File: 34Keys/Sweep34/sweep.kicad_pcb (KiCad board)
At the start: 2 copper layers, 110 x 88.6 mm, 21 parts, among them J1 MJ-4PP-9, SW10 SW_PUSH, SW11 SW_PUSH, SW12 SW_PUSH, SW14 SW_PUSH, SW15 SW_PUSH, SW16 SW_PUSH, SW17 SW_PUSH, SW18 SW_PUSH, SW2 SW_PUSH, SW20 SW_PUSH, SW21 SW_PUSH, SW3 SW_PUSH, SW4 SW_PUSH, SW5 SW_PUSH, SW6 SW_PUSH, SW8 SW_PUSH, SW9 SW_PUSH, U1 ProMicro

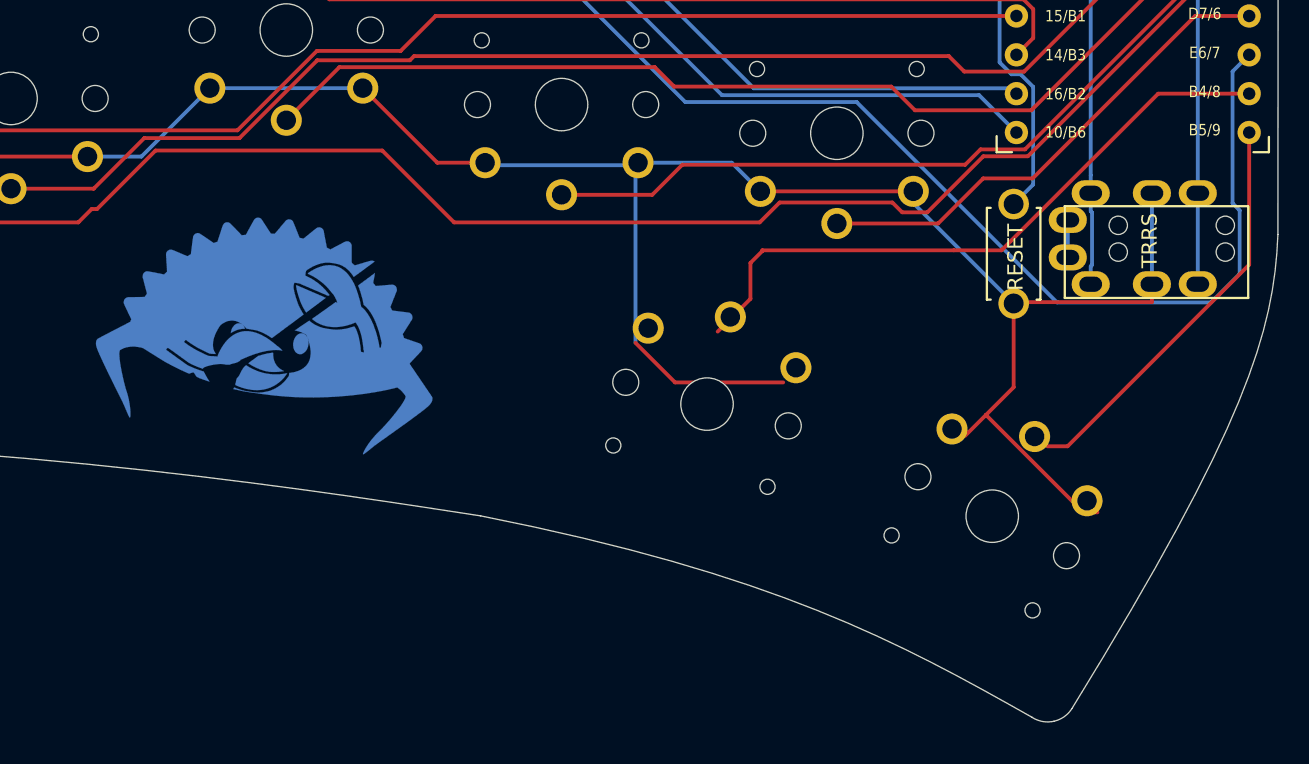
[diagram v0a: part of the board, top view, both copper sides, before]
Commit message: let's get these thumbs something like ferris
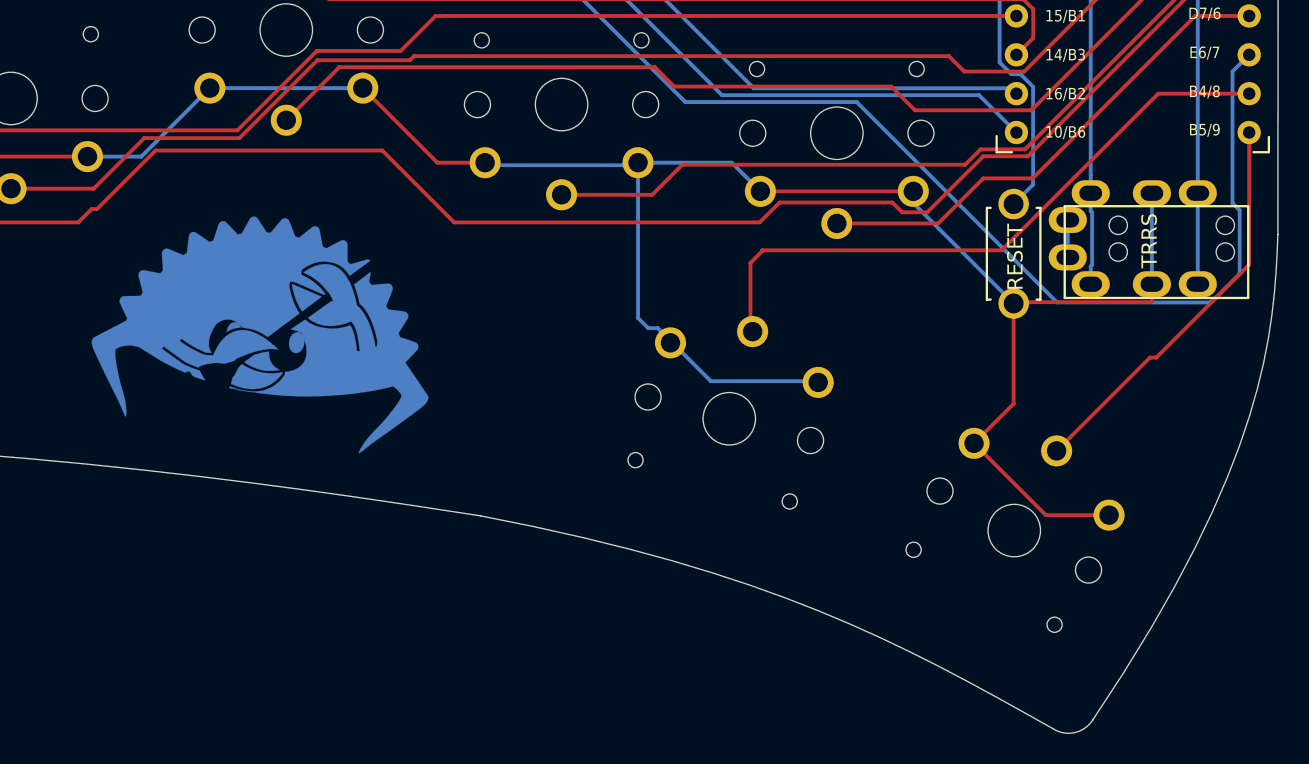
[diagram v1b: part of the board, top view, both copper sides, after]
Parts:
- moved SW20 1.74 mm to (109.0, 85.1)
- moved SW21 1.72 mm to (127.6, 92.4)
- moved G*** 0.28 mm to (79.8, 80.3)
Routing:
- net GND: track 393.6 -> 396.0 mm
- net Net-(U1-Pad11): track 42.6 -> 41.7 mm
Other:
- board size 110 x 88.6 mm -> 110 x 89.3 mm
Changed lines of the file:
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@@
   )
   (module Kailh:SW_PG1350_reversible_b2 (layer B.Cu)
-    (at 126.16 91.46 332)
+    (at 127.6 92.4 332)
     (descr "Kailh \"Choc\" PG1350 keyswitch, able to be mounted on front or back of PCB")
     (tags kailh,choc)
@@
   )
   (module Kailh:SW_PG1350_reversible_b2 (layer B.Cu)
-    (at 107.51 84.13 345)
+    (at 108.966 85.09 345)
     (descr "Kailh \"Choc\" PG1350 keyswitch, able to be mounted on front or back of PCB")
     (tags kailh,choc)
@@
   )
   (module Kailh:ferris_broom (layer B.Cu)
-    (at 80.07 80.4 171)
+    (at 79.8 80.33 171)
     (fp_text reference G*** (at 0 0 351) (layer B.SilkS) hide
       (effects (font (size 1.524 1.524) (thickness 0.3)) (justify mirror))
@@
   (gr_curve (pts (xy 144.87 34.010455) (xy 144.870889 33.819247) (xy 144.795513 33.637251) (xy 144.655943 33.499545)) (layer Edge.Cuts) (width 0.011328))
   (gr_curve (pts (xy 125.294806 23.859172) (xy 125.294794 23.580455) (xy 125.132917 23.327117) (xy 124.9 23.22)) (layer Edge.Cuts) (width 0.011328))
-  (gr_curve (pts (xy 130.186173 104.869608) (xy 130.675764 104.762323) (xy 131.102064 104.463579) (xy 131.37 104.04)) (layer Edge.Cuts) (width 0.011328))
-  (gr_curve (pts (xy 128.763902 104.611077) (xy 129.184419 104.883795) (xy 129.696582 104.976892) (xy 130.186173 104.869608)) (layer Edge.Cuts) (width 0.011328))
+  (gr_curve (pts (xy 131.55 105.61) (xy 132.039591 105.502715) (xy 132.465891 105.203971) (xy 132.73 104.79)) (layer Edge.Cuts) (width 0.011328))
+  (gr_curve (pts (xy 130.127729 105.351469) (xy 130.548246 105.624187) (xy 131.060409 105.717284) (xy 131.55 105.61)) (layer Edge.Cuts) (width 0.011328))
   (gr_curve (pts (xy 34.833624 84.713423) (xy 34.87005 85.754071) (xy 35.733715 86.573551) (xy 36.77484 86.555327)) (layer Edge.Cuts) (width 0.011328))
-  (gr_curve (pts (xy 128.763902 104.611077) (xy 120.073417 99.705624) (xy 111.98 95.25) (xy 92.71 91.44)) (layer Edge.Cuts) (width 0.011328))
+  (gr_curve (pts (xy 130.127729 105.351469) (xy 120.073417 99.705624) (xy 111.83 95.11) (xy 92.71 91.44)) (layer Edge.Cuts) (width 0.011328))
   (gr_line (start 125.3 31.44) (end 125.294806 23.859172) (layer Edge.Cuts) (width 0.011328))
   (gr_curve (pts (xy 124.9 23.22) (xy 111.07043 20.337524) (xy 96.846186 17.334305) (xy 84.254525 16.504695)) (layer Edge.Cuts) (width 0.011328))
@@
   (gr_curve (pts (xy 80.49 16.32) (xy 63.51 16.12) (xy 48.01 22.1) (xy 36.11 33.02)) (layer Edge.Cuts) (width 0.011328))
   (gr_line (start 144.87 34.010455) (end 144.84 73.04) (layer Edge.Cuts) (width 0.011328))
-  (gr_curve (pts (xy 131.37 104.04) (xy 142.702381 85.610668) (xy 144.590037 79.411298) (xy 144.84 73.04)) (layer Edge.Cuts) (width 0.011328))
+  (gr_curve (pts (xy 132.73 104.79) (xy 144.15 87.83) (xy 144.590037 79.411298) (xy 144.84 73.04)) (layer Edge.Cuts) (width 0.011328))
   (segment (start 142.9614 53.672) (end 139.966 53.672) (width 0.25) (layer F.Cu) (net 1))
   (segment (start 139.966 53.672) (end 128.7186 64.9194) (width 0.25) (layer F.Cu) (net 1))
@@
   (segment (start 49 80.175) (end 39 80.175) (width 0.25) (layer F.Cu) (net 5))
   (segment (start 102.8339 68.5111) (end 103 68.345) (width 0.25) (layer B.Cu) (net 5))
-  (segment (start 102.8339 80.1254) (end 102.8339 68.5111) (width 0.25) (layer B.Cu) (net 5))
   (segment (start 102.8339 68.5111) (end 93.1661 68.5111) (width 0.25) (layer B.Cu) (net 5))
   (segment (start 93.1661 68.5111) (end 93 68.345) (width 0.25) (layer B.Cu) (net 5))
@@
   (segment (start 88.2995 46.6395) (end 88.2995 46.47) (width 0.25) (layer B.Cu) (net 5))
   (segment (start 88.2995 46.47) (end 85 46.47) (width 0.25) (layer B.Cu) (net 5))
-  (segment (start 125.7506 84.8384) (end 124.3799 86.2091) (width 0.25) (layer F.Cu) (net 5))
-  (segment (start 127.56 77.55) (end 127.56 83.029) (width 0.25) (layer F.Cu) (net 5))
-  (segment (start 127.56 83.029) (end 125.7506 84.8384) (width 0.25) (layer F.Cu) (net 5))
-  (segment (start 125.7506 84.8384) (end 132.1213 91.2091) (width 0.25) (layer F.Cu) (net 5))
-  (segment (start 132.1213 91.2091) (end 133.0401 91.2091) (width 0.25) (layer F.Cu) (net 5))
   (segment (start 136.6 77.4653) (end 127.6447 77.4653) (width 0.25) (layer F.Cu) (net 5))
   (segment (start 127.6447 77.4653) (end 127.56 77.55) (width 0.25) (layer F.Cu) (net 5))
@@
   (segment (start 75 63.47) (end 70.525 67.945) (width 0.25) (layer B.Cu) (net 5))
   (segment (start 70.525 67.945) (end 67 67.945) (width 0.25) (layer B.Cu) (net 5))
-  (segment (start 112.4931 82.7136) (end 105.4221 82.7136) (width 0.25) (layer F.Cu) (net 5))
-  (segment (start 105.4221 82.7136) (end 102.8339 80.1254) (width 0.25) (layer F.Cu) (net 5))
   (segment (start 142.9614 43.512) (end 140.4214 40.972) (width 0.25) (layer F.Cu) (net 5))
   (segment (start 140.4214 40.972) (end 127.7414 40.972) (width 0.25) (layer F.Cu) (net 5))
@@
   (segment (start 136.6 76.29) (end 136.6 77.4653) (width 0.25) (layer F.Cu) (net 5))
   (segment (start 136.6 76.29) (end 136.6 70.34) (width 0.25) (layer B.Cu) (net 5))
+  (segment (start 103 78.501504) (end 103.663883 79.165387) (width 0.25) (layer B.Cu) (net 5))
+  (segment (start 103 68.345) (end 103 78.501504) (width 0.25) (layer B.Cu) (net 5))
+  (segment (start 127.56 84.106695) (end 124.969254 86.697441) (width 0.25) (layer F.Cu) (net 5))
+  (segment (start 127.56 77.55) (end 127.56 84.106695) (width 0.25) (layer F.Cu) (net 5))
+  (segment (start 129.66397 91.392157) (end 133.79873 91.392157) (width 0.25) (layer F.Cu) (net 5))
+  (segment (start 124.969254 86.697441) (end 129.66397 91.392157) (width 0.25) (layer F.Cu) (net 5))
+  (segment (start 107.762073 82.633577) (end 105.173883 80.045387) (width 0.25) (layer B.Cu) (net 5))
+  (segment (start 114.833142 82.633577) (end 107.762073 82.633577) (width 0.25) (layer B.Cu) (net 5))
+  (segment (start 104.293883 79.165387) (end 105.173883 80.045387) (width 0.25) (layer B.Cu) (net 5))
+  (segment (start 103.663883 79.165387) (end 104.293883 79.165387) (width 0.25) (layer B.Cu) (net 5))
   (segment (start 132.6 69.1647) (end 132.6 50.9106) (width 0.25) (layer B.Cu) (net 6))
   (segment (start 132.6 50.9106) (end 127.7414 46.052) (width 0.25) (layer B.Cu) (net 6))
@@
   (segment (start 108.4899 63.9299) (end 98 53.44) (width 0.25) (layer B.Cu) (net 21))
   (segment (start 142.9614 66.372) (end 142.9614 75.0149) (width 0.25) (layer F.Cu) (net 22))
-  (segment (start 142.9614 75.0149) (end 131.0858 86.8905) (width 0.25) (layer F.Cu) (net 22))
-  (segment (start 131.0858 86.8905) (end 129.76 86.8905) (width 0.25) (layer F.Cu) (net 22))
-  (segment (start 137.0102 63.832) (end 142.9614 63.832) (width 0.25) (layer F.Cu) (net 23))
-  (segment (start 127.4086 73.4336) (end 137.0102 63.832) (width 0.25) (layer F.Cu) (net 23))
-  (segment (start 110.35 77.24807) (end 108.207032 79.391038) (width 0.25) (layer F.Cu) (net 23))
+  (segment (start 142.9614 75.0149) (end 136.88815 81.08815) (width 0.25) (layer F.Cu) (net 22))
+  (segment (start 136.472341 81.08815) (end 130.369882 87.190609) (width 0.25) (layer F.Cu) (net 22))
+  (segment (start 136.88815 81.08815) (end 136.472341 81.08815) (width 0.25) (layer F.Cu) (net 22))
+  (segment (start 110.35 74.9) (end 110.35 79.114006) (width 0.25) (layer F.Cu) (net 23))
+  (segment (start 110.35 79.114006) (end 110.547032 79.311038) (width 0.25) (layer F.Cu) (net 23))
+  (segment (start 142.9614 63.832) (end 137.0102 63.832) (width 0.25) (layer F.Cu) (net 23))
   (segment (start 111.125 74.125) (end 110.35 74.9) (width 0.25) (layer F.Cu) (net 23))
+  (segment (start 137.0102 63.832) (end 126.7672 74.075) (width 0.25) (layer F.Cu) (net 23))
+  (segment (start 126.7672 74.075) (end 111.125 74.075) (width 0.25) (layer F.Cu) (net 23))
   (segment (start 111.125 74.075) (end 111.125 74.125) (width 0.25) (layer F.Cu) (net 23))
-  (segment (start 111.125 74.075) (end 123.65 74.075) (width 0.25) (layer F.Cu) (net 23))
-  (segment (start 110.35 74.9) (end 110.35 77.24807) (width 0.25) (layer F.Cu) (net 23))
-  (segment (start 126.7672 74.075) (end 126.8711 73.9711) (width 0.25) (layer F.Cu) (net 23))
-  (segment (start 123.65 74.075) (end 126.7672 74.075) (width 0.25) (layer F.Cu) (net 23))
-  (segment (start 126.8711 73.9711) (end 127.4086 73.4336) (width 0.25) (layer F.Cu) (net 23))
 )

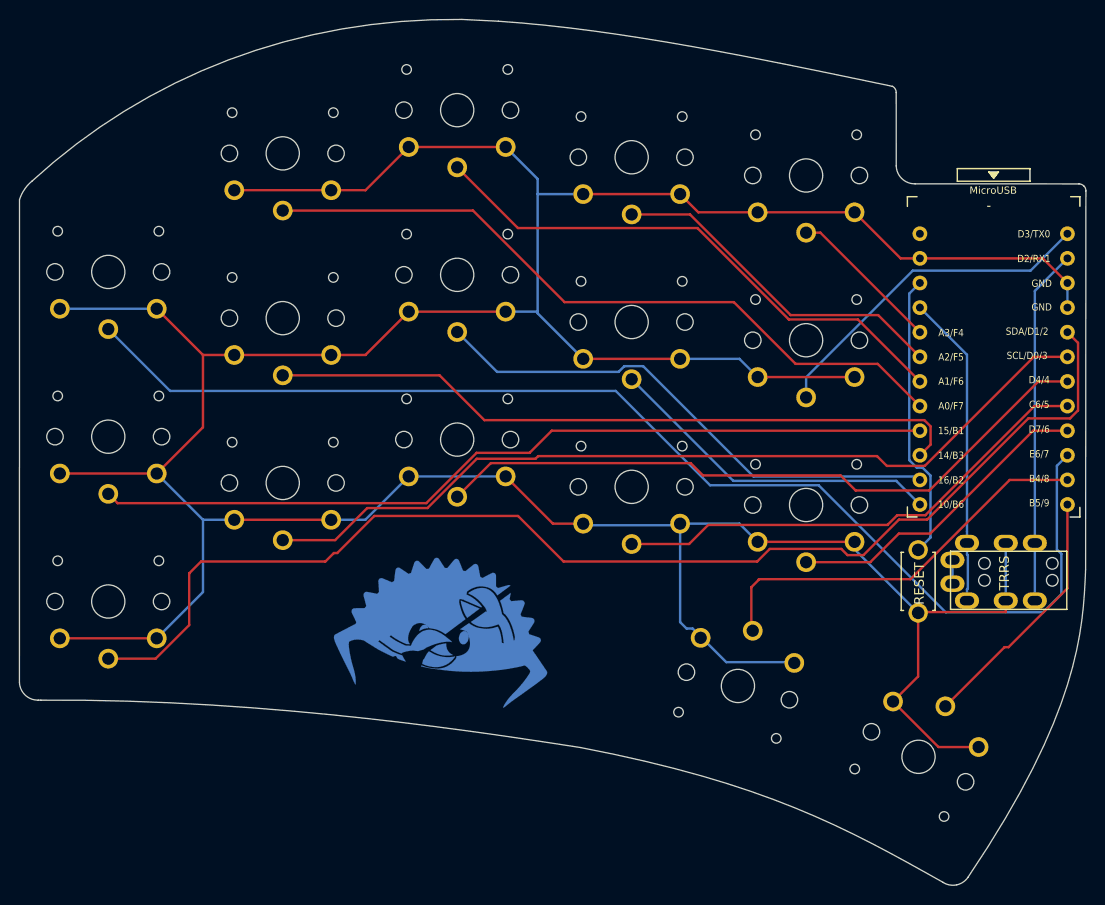
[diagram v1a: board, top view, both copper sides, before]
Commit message: curve changes
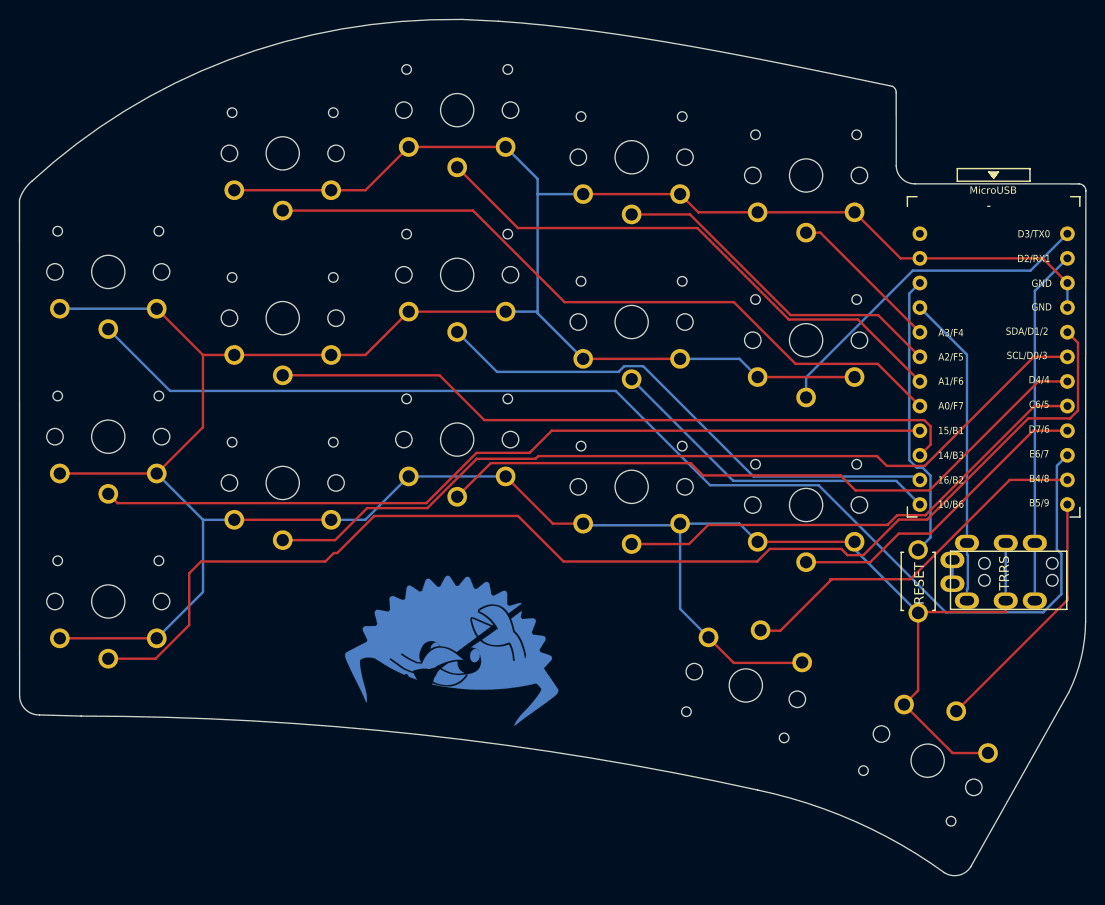
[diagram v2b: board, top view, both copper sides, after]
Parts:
- moved G*** 2.18 mm to (81.0, 82.2)
- moved SW21 1.02 mm to (128.5, 92.8), turned to 330 degrees
- moved SW20 0.82 mm to (109.8, 85.0)
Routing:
- net Net-(U1-Pad11): track 41.7 -> 38.3 mm
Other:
- board size 110 x 89.3 mm -> 110 x 88.3 mm
